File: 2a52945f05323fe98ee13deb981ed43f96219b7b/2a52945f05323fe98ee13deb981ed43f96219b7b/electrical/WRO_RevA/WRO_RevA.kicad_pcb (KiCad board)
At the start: 2 copper layers, 87.2 x 93.9 mm, 24 parts, among them J1 VCC, J3 TO_PI, J4 SERVO, J5 MOTOR, SW1 EXEC_PRGM, U1 ESP32-DEVKITC-32D, U2 ROB-14450, U3 BOB-12009, U4 MPU6050

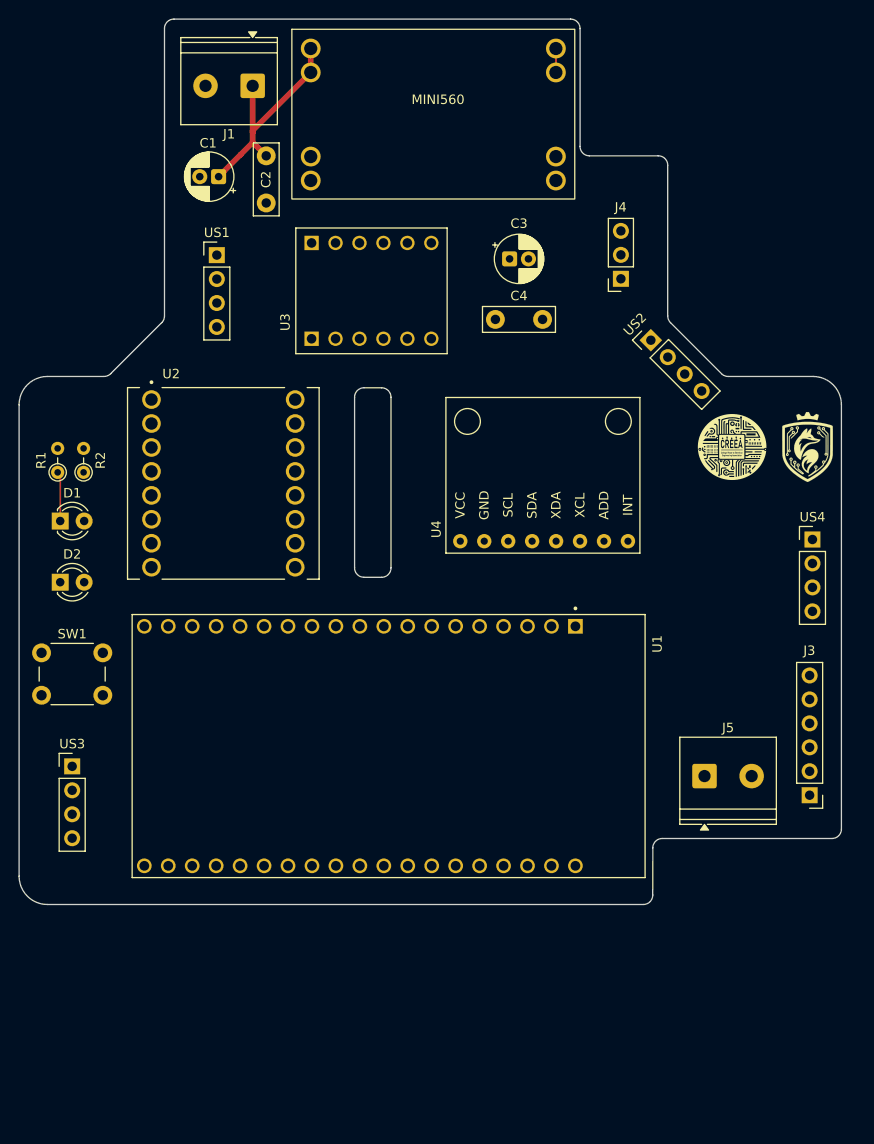
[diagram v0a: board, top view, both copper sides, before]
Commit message: finished
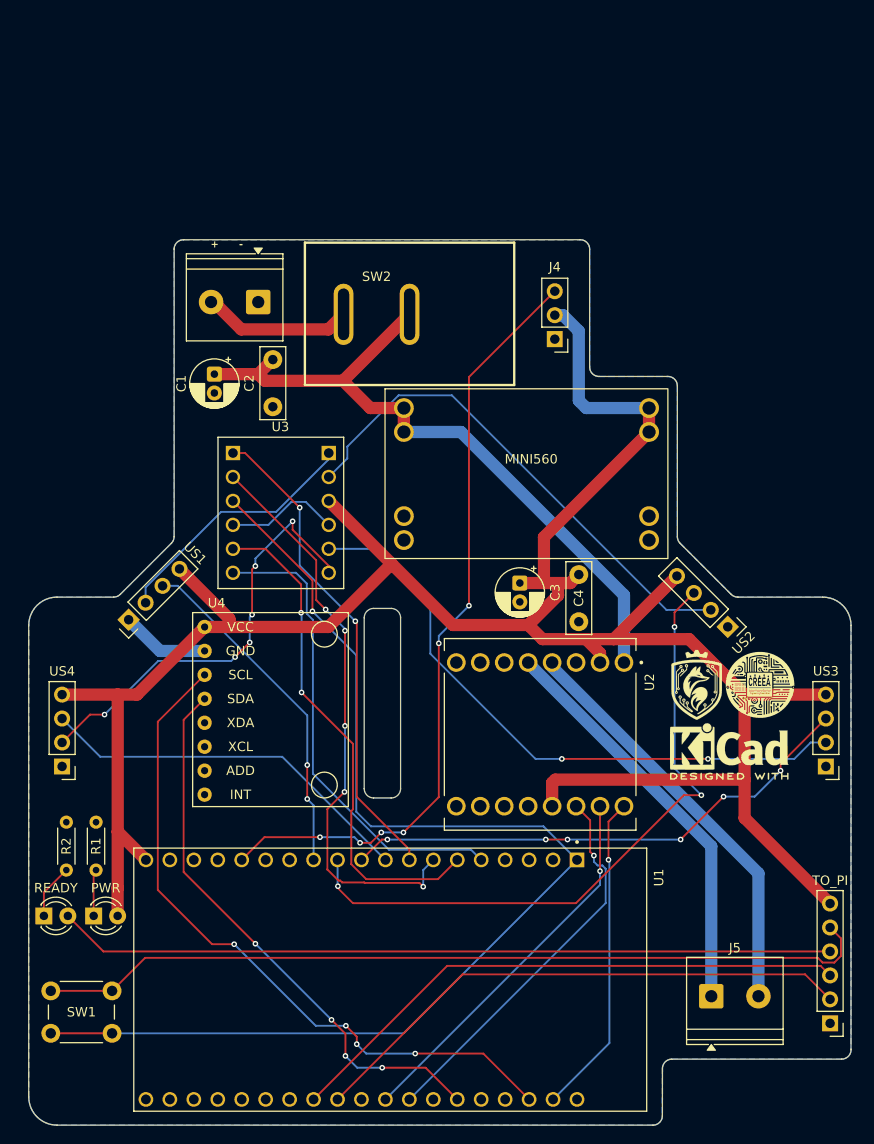
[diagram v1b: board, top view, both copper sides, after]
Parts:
- removed D1: PWR, LED_THT:LED_D3.0mm
- removed D2: READY, LED_THT:LED_D3.0mm
- removed J3: TO_PI, Connector_PinHeader_2.54mm:PinHeader_1x06_P2.54mm_Vertical
- added PWR: PWR, LED_THT:LED_D3.0mm, F.Cu at (109.1, 124.0)
- added READY: READY, LED_THT:LED_D3.0mm, F.Cu at (103.8, 124.0)
- added REF**: KiCad-Logo2_5mm_SilkScreen, Symbol:KiCad-Logo2_5mm_SilkScreen, F.Cu at (176.5, 106.6)
- added SW2: PWR, EasyEDA:SW-TH_L22.2-W15.0-P7.00_KCD1-2P-P, F.Cu at (139.1, 60.2)
- added TO_PI: TO_PI, Connector_PinHeader_2.54mm:PinHeader_1x06_P2.54mm_Vertical, F.Cu at (187.2, 135.4)
- J4: footprint Connector_PinSocket_2.54mm:PinSocket_1x03_P2.54mm_Vertical -> Connector_PinHeader_2.54mm:PinHeader_1x03_P2.54mm_Vertical
- R1, R2: footprint Resistor_THT:R_Axial_DIN0204_L3.6mm_D1.6mm_P2.54mm_Vertical -> Resistor_THT:R_Axial_DIN0204_L3.6mm_D1.6mm_P5.08mm_Horizontal
- moved US4 83.1 mm to (105.8, 108.2), turned to 180 degrees
- moved US3 79.9 mm to (186.8, 108.2), turned to 180 degrees
- moved U4 52.3 mm to (120.9, 111.2), turned to 0 degrees
- moved U2 42.9 mm to (156.4, 104.8), turned to -90 degrees
- moved R1 42.4 mm to (109.3, 119.2)
- moved R2 42.2 mm to (106.2, 119.2)
- moved SW1 41.0 mm to (111.0, 136.5), turned to 180 degrees
- moved US1 39.8 mm to (112.8, 92.6), turned to 135 degrees
- moved MINI560 39.4 mm to (155.0, 77.2)
- moved C3 34.4 mm to (154.3, 88.8), turned to -90 degrees
- moved US2 31.5 mm to (176.3, 93.4), turned to -135 degrees
- moved C4 28.5 mm to (160.6, 87.8), turned to -90 degrees
- moved G*** 27.8 mm to (173.1, 99.7)
- moved U3 25.4 mm to (128.9, 81.3), turned to 0 degrees
- moved G*** 25.4 mm to (179.8, 99.5)
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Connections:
- J1 pad 1: +11.2V -> GND
- J1 pad 2: GND -> Net-(J1-Pin_2)
- U1 pad J2-13: STBY -> unconnected-(U1-IO12-PadJ2-13)
- U2 pad 13: STBY -> +5V
- US2 pad 3: unconnected-(US2-Pin_3-Pad3) -> TRIG2
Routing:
- net +5V: track 2.54 -> 253.4 mm
- net +3V3: track 0.00 -> 127.3 mm, vias 0 -> 1
- net PRGM: track 0.00 -> 89.2 mm
- net SERVO: track 0.00 -> 83.2 mm, vias 0 -> 6
- net READY: track 0.00 -> 82.4 mm
- net SCL: track 0.00 -> 73.9 mm, vias 0 -> 4
- net TRIG2: track 0.00 -> 70.5 mm, vias 0 -> 3
- net ECHO3: track 0.00 -> 66.2 mm, vias 0 -> 2
- net ECHO2_L: track 0.00 -> 61.7 mm, vias 0 -> 5
- net RX: track 0.00 -> 61.1 mm
- net SDA: track 0.00 -> 59.6 mm, vias 0 -> 4
- net TX: track 0.00 -> 58.8 mm
- net TRIG3: track 0.00 -> 55.9 mm, vias 0 -> 6
- net ECHO2: track 0.00 -> 54.3 mm
- net ECHO3_L: track 0.00 -> 53.6 mm, vias 0 -> 2
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- added copper zone on B.Cu, net GND
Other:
- board text added: "+ -"
